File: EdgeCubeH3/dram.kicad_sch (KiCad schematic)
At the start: 15 parts, among them U2 K4B4G1646Q

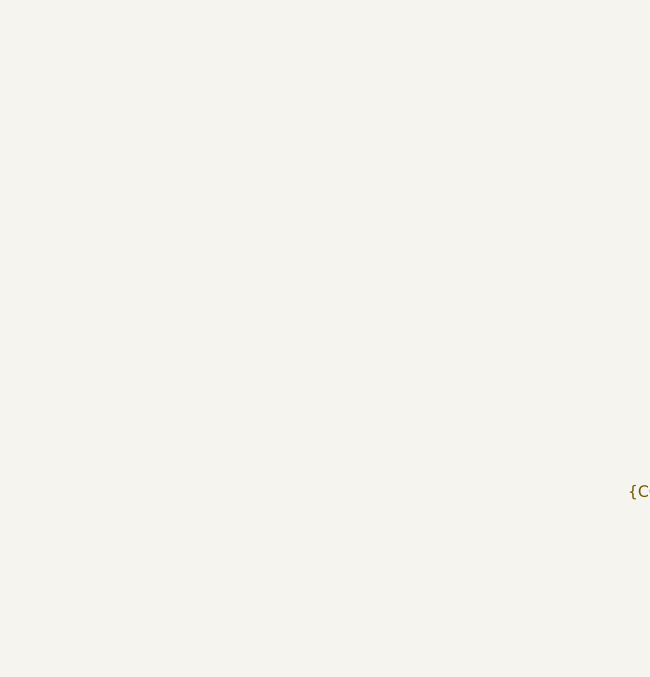
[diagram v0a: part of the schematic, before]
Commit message: Schematic update, PCB started
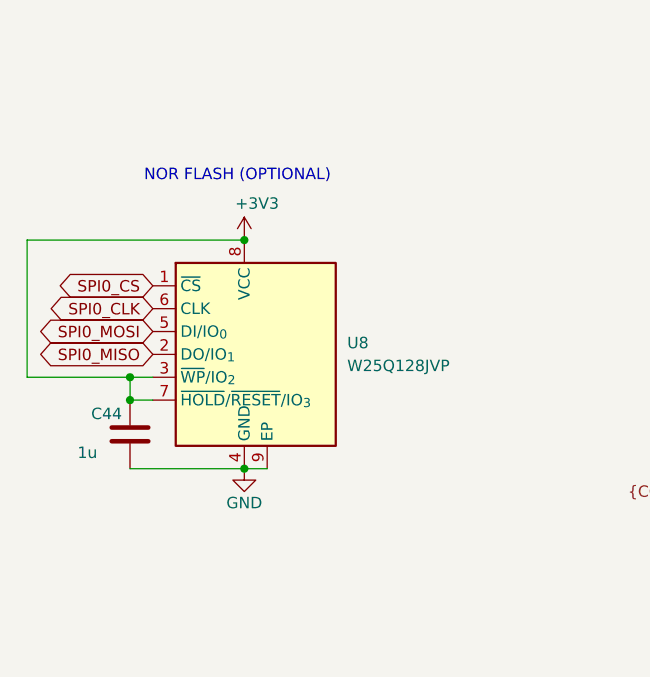
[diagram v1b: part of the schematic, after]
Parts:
- added C44: 1u, Capacitor_SMD:C_0603_1608Metric, symbol Device:C
- added U8: W25Q128JVP, Package_SON:WSON-8-1EP_6x5mm_P1.27mm_EP3.4x4.3mm, symbol Memory_Flash:W25Q128JVP
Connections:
- net GND: now also C44.2, U8.4 (GND), U8.9 (EP)
- new net +3V3: C44.1, U8.3 (~{WP}/IO_{2}), U8.7 (~{HOLD}/~{RESET}/IO_{3}), U8.8 (VCC)
- new net SPI0_CLK: U8.6 (CLK)
- new net SPI0_CS: U8.1 (~{CS})
- new net SPI0_MISO: U8.2 (DO/IO_{1})
- new net SPI0_MOSI: U8.5 (DI/IO_{0})
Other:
- note added: "NOR FLASH (OPTIONAL)"
